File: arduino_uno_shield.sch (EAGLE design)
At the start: 12 parts

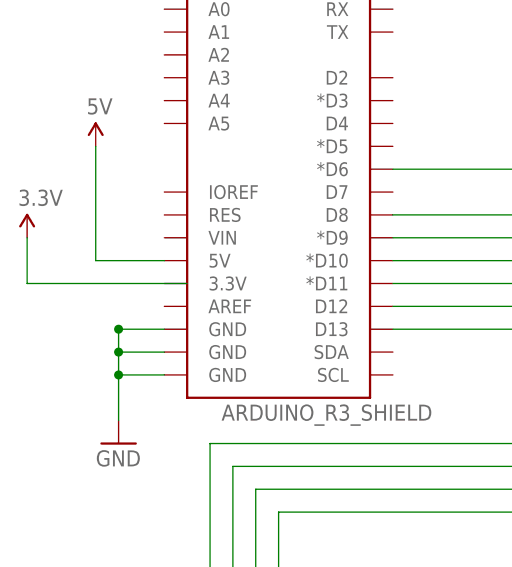
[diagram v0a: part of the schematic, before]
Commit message: first attempt at board layout
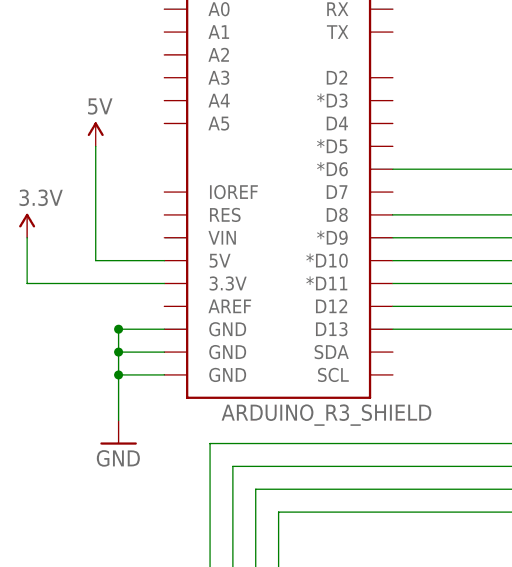
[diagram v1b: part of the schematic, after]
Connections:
- net 3.3V: now also U$1.3.3V
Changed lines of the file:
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@@
 <pinref part="SUPPLY1" gate="G$1" pin="3.3V"/>
 <wire x1="-157.48" y1="66.04" x2="-157.48" y2="60.96" width="0.1524" layer="91"/>
-<wire x1="-157.48" y1="60.96" x2="-139.7" y2="60.96" width="0.1524" layer="91"/>
+<pinref part="U$1" gate="G$1" pin="3.3V"/>
+<wire x1="-157.48" y1="60.96" x2="-142.24" y2="60.96" width="0.1524" layer="91"/>
 </segment>
 </net>

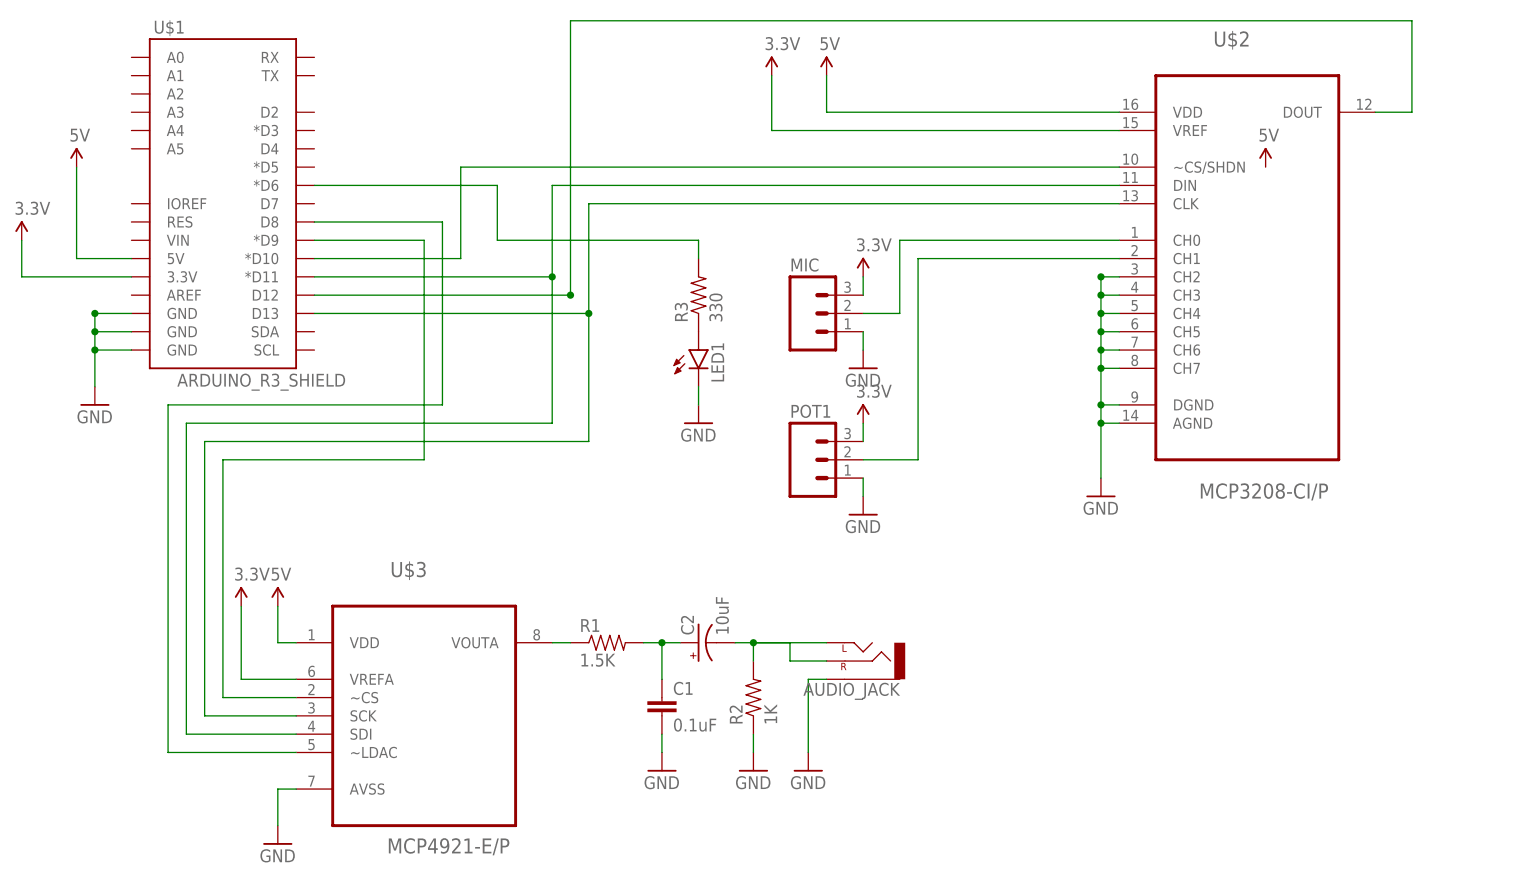
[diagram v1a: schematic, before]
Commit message: removed board
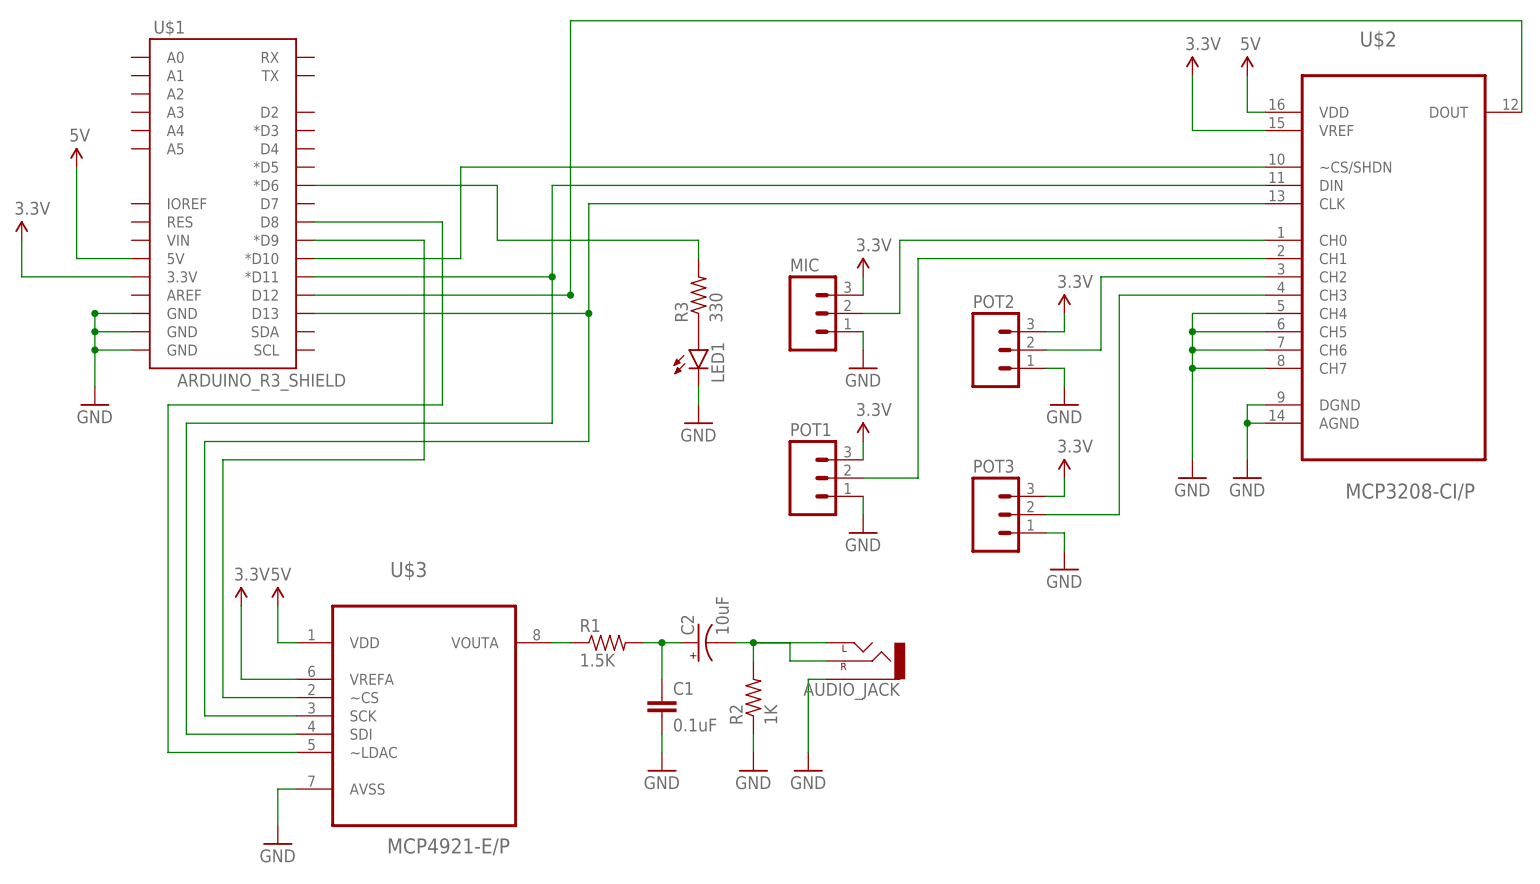
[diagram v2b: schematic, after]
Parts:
- added POT2, POT3: (no value), SparkFun-Connectors:M03PTH
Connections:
- new net N$14: POT2.2, U$2.CH2
- new net N$15: POT3.2, U$2.CH3
- net 3.3V: now also POT2.3, POT3.3
- net GND: now also POT2.1, POT3.1; no longer U$2.CH2, U$2.CH3
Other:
- moved on the sheet: POT1, U$2
